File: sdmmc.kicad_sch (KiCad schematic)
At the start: 18 parts, among them J4 Micro_SD_Card_Det2

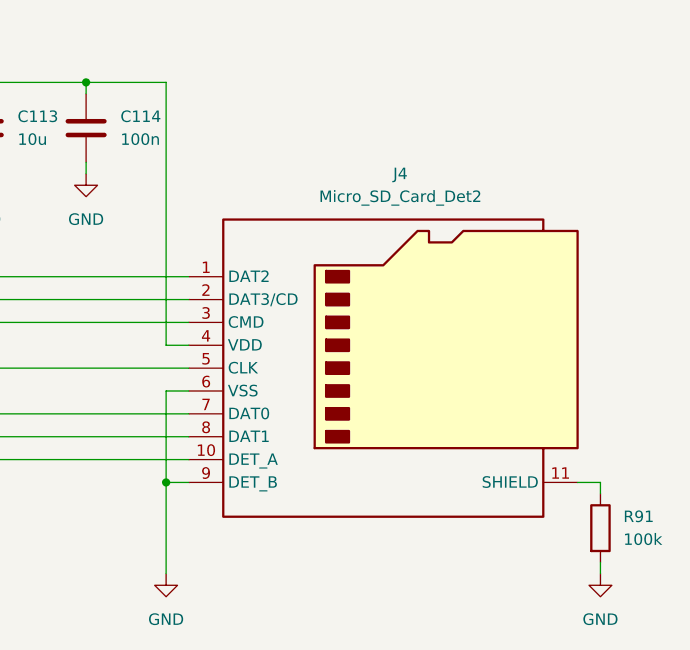
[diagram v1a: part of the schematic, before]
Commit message: many stuffs
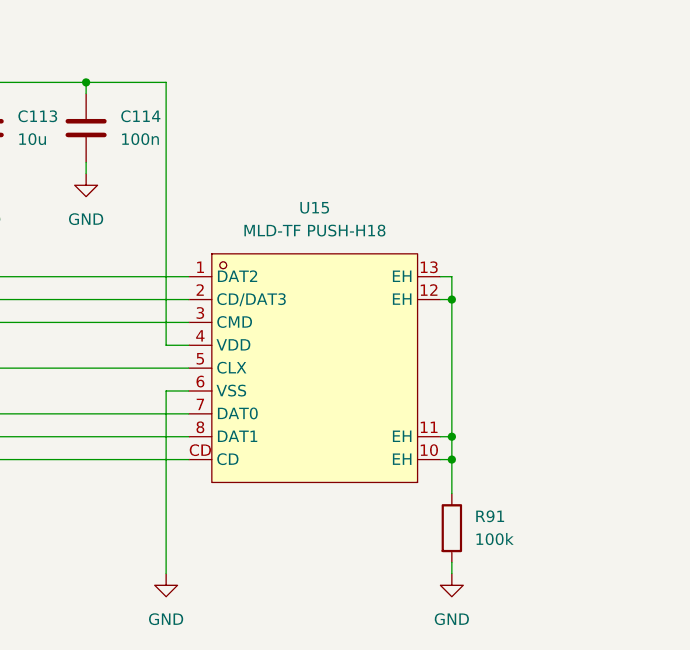
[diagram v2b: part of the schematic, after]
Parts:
- removed J4: Micro_SD_Card_Det2, Connector_Card:microSD_HC_Hirose_DM3AT-SF-PEJM5, symbol Connector:Micro_SD_Card_Det2
- added U15: MLD-TF PUSH-H18, C52750848:SD-SMD_MLD-TF-PUSH-H18, symbol C52750848:MLD-TFPUSH-H18
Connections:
- net +3.3V: now also U15.4 (VDD)
- net GND: now also U15.6 (VSS)
- net MMC.SDCD: now also U15.CD
- net MMC.SDCK: now also U15.5 (CLX)
- net MMC.SDCMD: now also U15.3 (CMD)
- net MMC.SDDAT0: now also U15.7 (DAT0)
- net MMC.SDDAT1: now also U15.8 (DAT1)
- net MMC.SDDAT2: now also U15.1 (DAT2)
- net MMC.SDDAT3: now also U15.2 (CD/DAT3)
- net at R91.1: now also U15.10 (EH), U15.11 (EH), U15.12 (EH), U15.13 (EH)
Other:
- moved on the sheet: R91
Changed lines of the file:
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@@
 	)
 	(junction
-		(at 204.47 104.14)
+		(at 153.67 86.36)
 		(diameter 0)
 		(color 0 0 0 0)
 	)
 	(junction
-		(at 153.67 86.36)
+		(at 236.22 99.06)
 		(diameter 0)
 		(color 0 0 0 0)
@@
 	)
 	(junction
+		(at 236.22 101.6)
+		(diameter 0)
+		(color 0 0 0 0)
+	)
+	(junction
 		(at 149.86 86.36)
 		(diameter 0)
@@
 	)
 	(junction
+		(at 236.22 83.82)
+		(diameter 0)
+		(color 0 0 0 0)
+	)
+	(junction
 		(at 118.11 101.6)
 		(diameter 0)
@@
 	(wire
 		(pts
-			(xy 204.47 93.98) (xy 204.47 104.14)
+			(xy 204.47 93.98) (xy 204.47 114.3)
 		)
 		(stroke
@@
 	(wire
 		(pts
+			(xy 236.22 101.6) (xy 236.22 105.41)
+		)
+		(stroke
+			(width 0)
+			(type default)
+		)
+	)
+	(wire
+		(pts
 			(xy 180.34 59.69) (xy 184.15 59.69)
 		)
@@
 	(wire
 		(pts
+			(xy 236.22 99.06) (xy 234.95 99.06)
+		)
+		(stroke
+			(width 0)
+			(type default)
+		)
+	)
+	(wire
+		(pts
 			(xy 153.67 86.36) (xy 207.01 86.36)
 		)
@@
 	(wire
 		(pts
-			(xy 252.73 105.41) (xy 252.73 104.14)
+			(xy 140.97 64.77) (xy 149.86 64.77)
 		)
 		(stroke
@@
 	(wire
 		(pts
-			(xy 140.97 64.77) (xy 149.86 64.77)
+			(xy 236.22 81.28) (xy 236.22 83.82)
 		)
 		(stroke
@@
 	(wire
 		(pts
-			(xy 252.73 113.03) (xy 252.73 114.3)
+			(xy 236.22 113.03) (xy 236.22 114.3)
+		)
+		(stroke
+			(width 0)
+			(type default)
+		)
+	)
+	(wire
+		(pts
+			(xy 234.95 81.28) (xy 236.22 81.28)
 		)
 		(stroke
@@
 	(wire
 		(pts
-			(xy 204.47 104.14) (xy 207.01 104.14)
-		)
-		(stroke
-			(width 0)
-			(type default)
-		)
-	)
-	(wire
-		(pts
 			(xy 100.33 96.52) (xy 132.08 96.52)
 		)
@@
 	(wire
 		(pts
+			(xy 234.95 83.82) (xy 236.22 83.82)
+		)
+		(stroke
+			(width 0)
+			(type default)
+		)
+	)
+	(wire
+		(pts
 			(xy 114.3 73.66) (xy 114.3 101.6)
 		)
@@
 	(wire
 		(pts
-			(xy 250.19 104.14) (xy 252.73 104.14)
+			(xy 234.95 101.6) (xy 236.22 101.6)
 		)
 		(stroke
@@
 	(wire
 		(pts
-			(xy 135.89 96.52) (xy 207.01 96.52)
+			(xy 236.22 101.6) (xy 236.22 99.06)
 		)
 		(stroke
@@
 	(wire
 		(pts
-			(xy 162.56 83.82) (xy 207.01 83.82)
+			(xy 236.22 83.82) (xy 236.22 99.06)
 		)
 		(stroke
@@
 	(wire
 		(pts
-			(xy 135.89 113.03) (xy 135.89 114.3)
+			(xy 135.89 96.52) (xy 207.01 96.52)
 		)
 		(stroke
@@
 	(wire
 		(pts
-			(xy 123.19 99.06) (xy 127 99.06)
+			(xy 162.56 83.82) (xy 207.01 83.82)
 		)
 		(stroke
@@
 	(wire
 		(pts
-			(xy 204.47 104.14) (xy 204.47 114.3)
+			(xy 135.89 113.03) (xy 135.89 114.3)
+		)
+		(stroke
+			(width 0)
+			(type default)
+		)
+	)
+	(wire
+		(pts
+			(xy 123.19 99.06) (xy 127 99.06)
 		)
 		(stroke
@@
 	)
 	(symbol
+		(lib_id "C52750848:MLD-TFPUSH-H18")
+		(at 219.71 93.98 0)
+		(unit 1)
+		(body_style 1)
+		(exclude_from_sim no)
+		(in_bom yes)
+		(on_board yes)
+		(in_pos_files yes)
+		(dnp no)
+		(fields_autoplaced yes)
+		(property "Reference" "U15"
+			(at 220.98 73.66 0)
+			(show_name no)
+			(do_not_autoplace no)
+			(effects
+				(font
+					(size 1.27 1.27)
+				)
+			)
+		)
+		(property "Value" "MLD-TF PUSH-H18"
+			(at 220.98 76.2 0)
+			(show_name no)
+			(do_not_autoplace no)
+			(effects
+				(font
+					(size 1.27 1.27)
+				)
+			)
+		)
+		(property "Footprint" "C52750848:SD-SMD_MLD-TF-PUSH-H18"
+			(at 219.71 109.22 0)
+			(hide yes)
+			(show_name no)
+			(do_not_autoplace no)
+			(effects
+				(font
+					(size 1.27 1.27)
+				)
+			)
+		)
+		(property "Datasheet" ""
+			(at 219.71 93.98 0)
+			(hide yes)
+			(show_name no)
+			(do_not_autoplace no)
+			(effects
+				(font
+					(size 1.27 1.27)
+				)
+			)
+		)
+		(property "Description" ""
+			(at 219.71 93.98 0)
+			(hide yes)
+			(show_name no)
+			(do_not_autoplace no)
+			(effects
+				(font
+					(size 1.27 1.27)
+				)
+			)
+		)
+		(property "LCSC Part" "C52750848"
+			(at 219.71 111.76 0)
+			(hide yes)
+			(show_name no)
+			(do_not_autoplace no)
+			(effects
+				(font
+					(size 1.27 1.27)
+				)
+			)
+		)
+		(pin "CD"
+		)
+		(pin "11"
+		)
+		(pin "13"
+		)
+		(pin "10"
+		)
+		(pin "12"
+		)
+		(pin "8"
+		)
+		(pin "7"
+		)
+		(pin "6"
+		)
+		(pin "5"
+		)
+		(pin "2"
+		)
+		(pin "4"
+		)
+		(pin "1"
+		)
+		(pin "3"
+		)
+		(instances
+			(project "netdaq"
+				(path "/2970f661-65ab-4e2b-aeda-d76d1044f2b8/1813fba9-8b3b-4d19-ab19-e743aa636a8b"
+					(reference "U15")
+					(unit 1)
+				)
+			)
+		)
+	)
+	(symbol
 		(lib_id "Device:R")
 		(at 132.08 69.85 0)
@@
 	(symbol
 		(lib_id "power:GND")
-		(at 252.73 114.3 0)
+		(at 236.22 114.3 0)
 		(unit 1)
 		(body_style 1)
@@
 		(fields_autoplaced yes)
 		(property "Reference" "#PWR0199"
-			(at 252.73 120.65 0)
+			(at 236.22 120.65 0)
 			(hide yes)
 			(show_name no)
@@
 		)
 		(property "Value" "GND"
-			(at 252.73 119.38 0)
+			(at 236.22 119.38 0)
 			(show_name no)
 			(do_not_autoplace no)
@@
 		)
 		(property "Footprint" ""
-			(at 252.73 114.3 0)
+			(at 236.22 114.3 0)
 			(hide yes)
 			(show_name no)
@@
 		)
 		(property "Datasheet" ""
-			(at 252.73 114.3 0)
+			(at 236.22 114.3 0)
 			(hide yes)
 			(show_name no)
@@
 		)
 		(property "Description" "Power symbol creates a global label with name \"GND\" , ground"
-			(at 252.73 114.3 0)
+			(at 236.22 114.3 0)
 			(hide yes)
 			(show_name no)
@@
 	)
 	(symbol
-		(lib_id "Connector:Micro_SD_Card_Det2")
-		(at 229.87 91.44 0)
-		(unit 1)
-		(body_style 1)
-		(exclude_from_sim no)
-		(in_bom yes)
-		(on_board yes)
-		(in_pos_files yes)
-		(dnp no)
-		(fields_autoplaced yes)
-		(property "Reference" "J4"
-			(at 230.505 69.85 0)
-			(show_name no)
-			(do_not_autoplace no)
-			(effects
-				(font
-					(size 1.27 1.27)
-				)
-			)
-		)
-		(property "Value" "Micro_SD_Card_Det2"
-			(at 230.505 72.39 0)
-			(show_name no)
-			(do_not_autoplace no)
-			(effects
-				(font
-					(size 1.27 1.27)
-				)
-			)
-		)
-		(property "Footprint" "Connector_Card:microSD_HC_Hirose_DM3AT-SF-PEJM5"
-			(at 281.94 73.66 0)
-			(hide yes)
-			(show_name no)
-			(do_not_autoplace no)
-			(effects
-				(font
-					(size 1.27 1.27)
-				)
-			)
-		)
-		(property "Datasheet" "https://www.hirose.com/en/product/document?clcode=&productname=&series=DM3&documenttype=Catalog&lang=en&documentid=D49662_en"
-			(at 232.41 88.9 0)
-			(hide yes)
-			(show_name no)
-			(do_not_autoplace no)
-			(effects
-				(font
-					(size 1.27 1.27)
-				)
-			)
-		)
-		(property "Description" "Micro SD Card Socket with two card detection pins"
-			(at 229.87 91.44 0)
-			(hide yes)
-			(show_name no)
-			(do_not_autoplace no)
-			(effects
-				(font
-					(size 1.27 1.27)
-				)
-			)
-		)
-		(pin "9"
-		)
-		(pin "8"
-		)
-		(pin "6"
-		)
-		(pin "7"
-		)
-		(pin "5"
-		)
-		(pin "4"
-		)
-		(pin "10"
-		)
-		(pin "3"
-		)
-		(pin "11"
-		)
-		(pin "1"
-		)
-		(pin "2"
-		)
-		(instances
-			(project "netdaq"
-				(path "/2970f661-65ab-4e2b-aeda-d76d1044f2b8/1813fba9-8b3b-4d19-ab19-e743aa636a8b"
-					(reference "J4")
-					(unit 1)
-				)
-			)
-		)
-	)
-	(symbol
 		(lib_id "power:GND")
 		(at 118.11 114.3 0)
@@
 	(symbol
 		(lib_id "Device:R")
-		(at 252.73 109.22 0)
+		(at 236.22 109.22 0)
 		(unit 1)
 		(body_style 1)
@@
 		(fields_autoplaced yes)
 		(property "Reference" "R91"
-			(at 255.27 107.9499 0)
+			(at 238.76 107.9499 0)
 			(show_name no)
 			(do_not_autoplace no)
@@
 		)
 		(property "Value" "100k"
-			(at 255.27 110.4899 0)
+			(at 238.76 110.4899 0)
 			(show_name no)
 			(do_not_autoplace no)
@@
 		)
 		(property "Footprint" "Resistor_SMD:R_0402_1005Metric"
-			(at 250.952 109.22 90)
+			(at 234.442 109.22 90)
 			(hide yes)
 			(show_name no)
@@
 		)
 		(property "Datasheet" ""
-			(at 252.73 109.22 0)
+			(at 236.22 109.22 0)
 			(hide yes)
 			(show_name no)
@@
 		)
 		(property "Description" "Resistor"
-			(at 252.73 109.22 0)
+			(at 236.22 109.22 0)
 			(hide yes)
 			(show_name no)
